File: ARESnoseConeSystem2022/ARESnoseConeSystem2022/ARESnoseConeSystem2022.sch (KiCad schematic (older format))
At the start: 14 parts, among them J1 436500200, J2 436500200, J3 BMP390_Headers, J4 ICM20948_Headers, J5 GPS_Headers1, J6 Transmitter_Headers1, J7 Conn_01x08, J8 Transmitter_Headers2, U1 L7805, U2 Teensy4.1

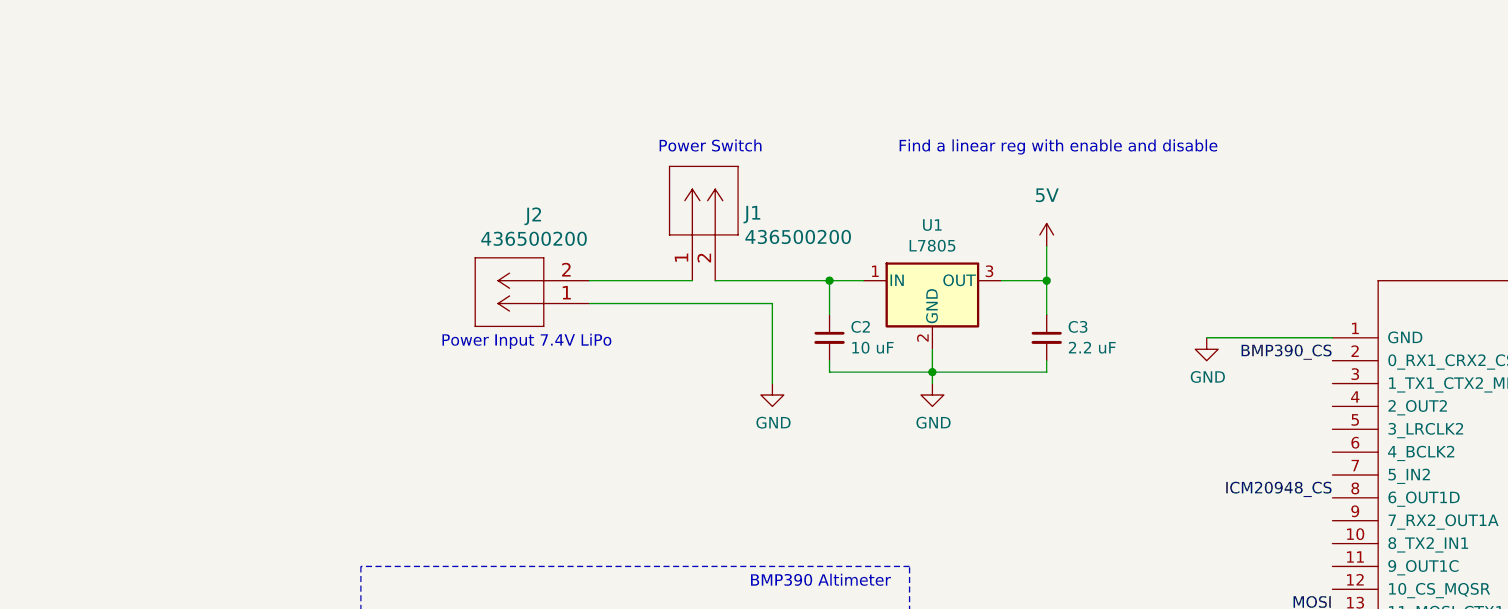
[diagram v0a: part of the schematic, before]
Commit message: Better regulator
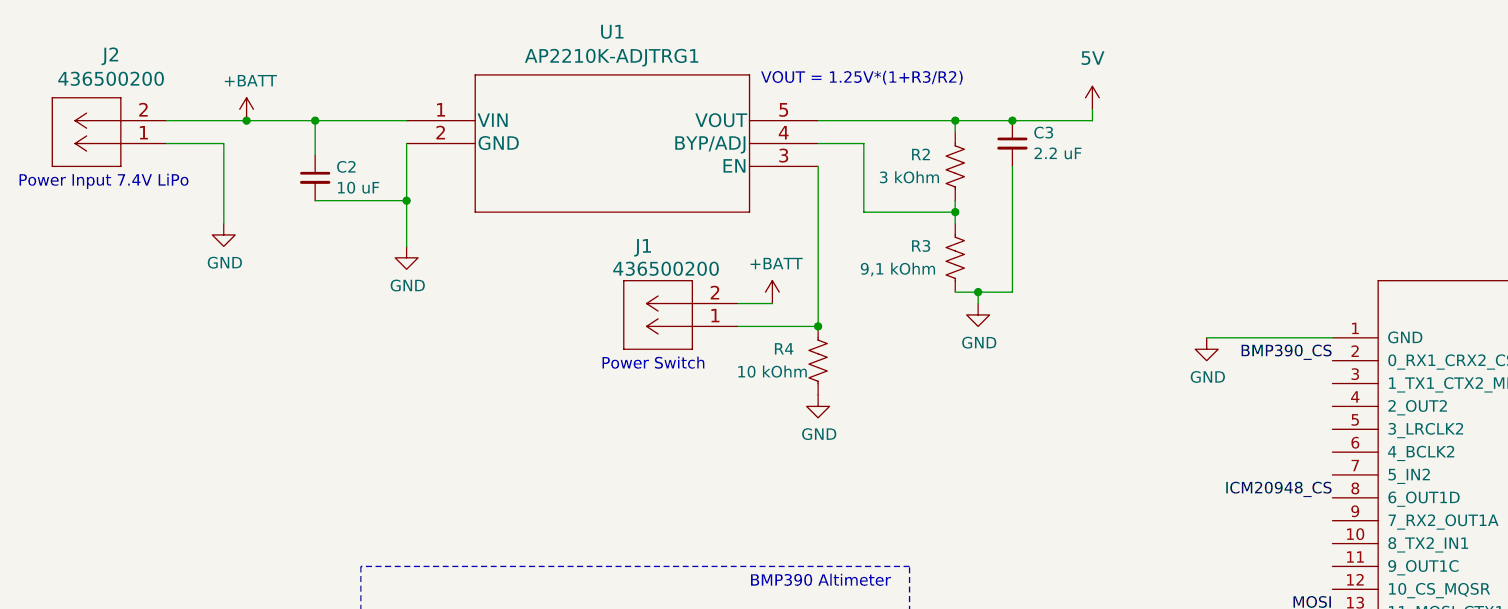
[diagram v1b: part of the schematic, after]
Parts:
- removed U1: L7805, Package_TO_SOT_THT:TO-220-3_Vertical, symbol Regulator_Linear:L7805
- added R2: 3 kOhm, Resistor_SMD:R_0805_2012Metric_Pad1.15x1.40mm_HandSolder, symbol Device:R_US
- added R3: 9,1 kOhm, Resistor_SMD:R_0805_2012Metric_Pad1.15x1.40mm_HandSolder, symbol Device:R_US
- added R4: 10 kOhm, Resistor_SMD:R_0805_2012Metric_Pad1.15x1.40mm_HandSolder, symbol Device:R_US
- added U1: AP2210K-ADJTRG1, SOT-23-5_DIO, symbol 5V-Reg:AP2210K-ADJTRG1
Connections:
- net GND: now also R3.2, R4.2, U1.2 (GND)
- net +BATT: now reaches C2.1, J1.2
- net +BATT: now also J2.2, U1.1 (VIN)
- net at C3.1: now also R2.1, U1.5 (VOUT)
- net at J1.1: now also R4.1, U1.3 (EN); no longer J2.2
- new net: R2.2, R3.1, U1.4 (BYP/ADJ)
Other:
- note added: "VOUT = 1.25V*(1+R3/R2)"
- note removed: "Find a linear reg with enable and disable"
- moved on the sheet: C2, C3, J1, J2
